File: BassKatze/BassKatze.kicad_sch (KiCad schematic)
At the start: 42 parts, among them U1 ESP32-WROOM-32D

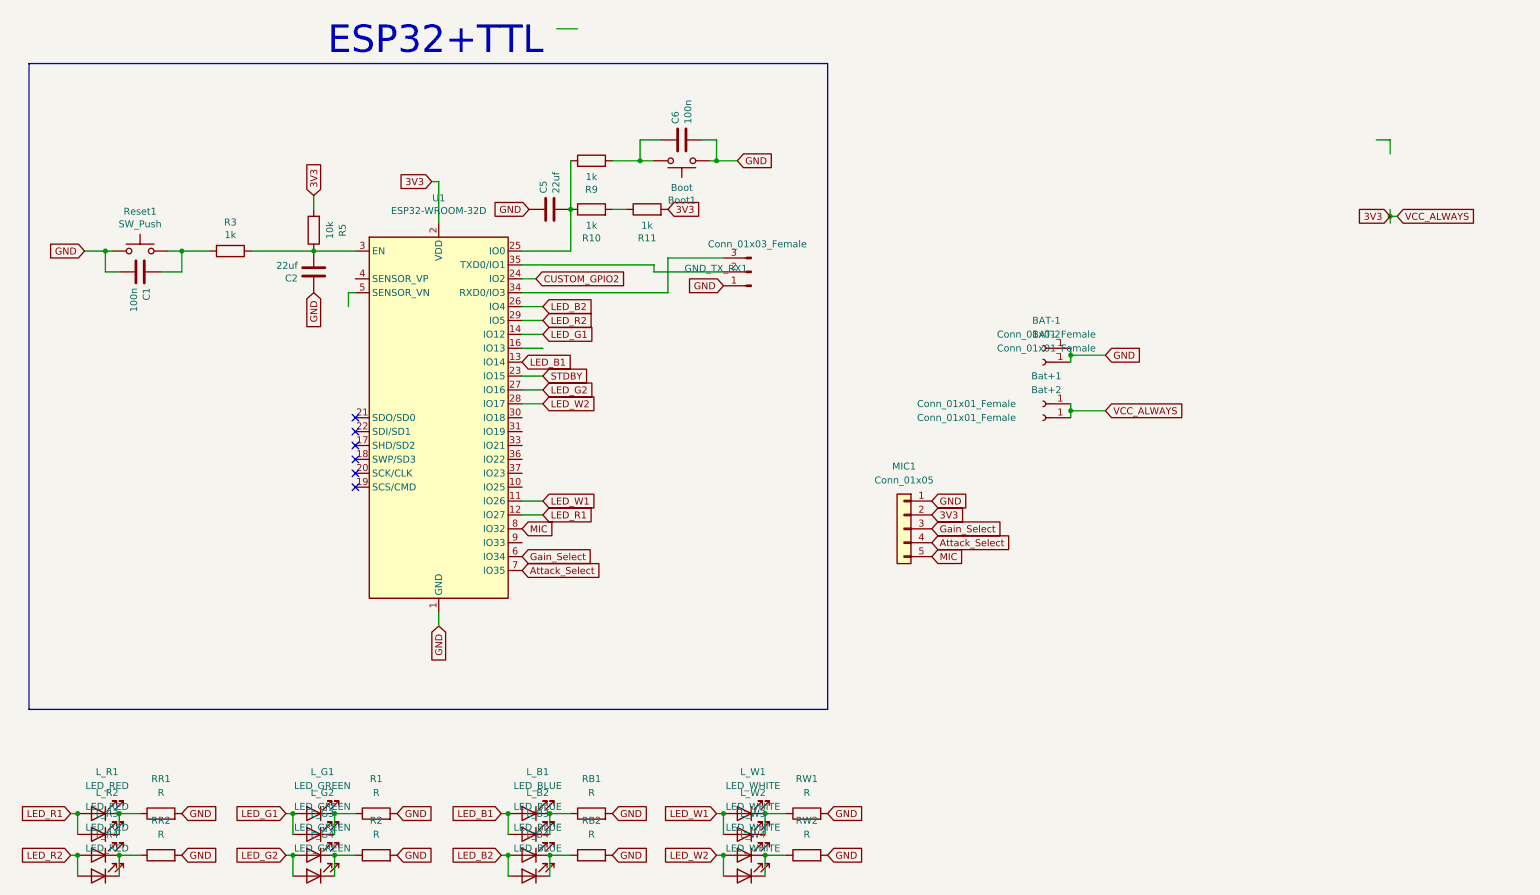
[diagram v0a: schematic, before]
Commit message: esp32 version
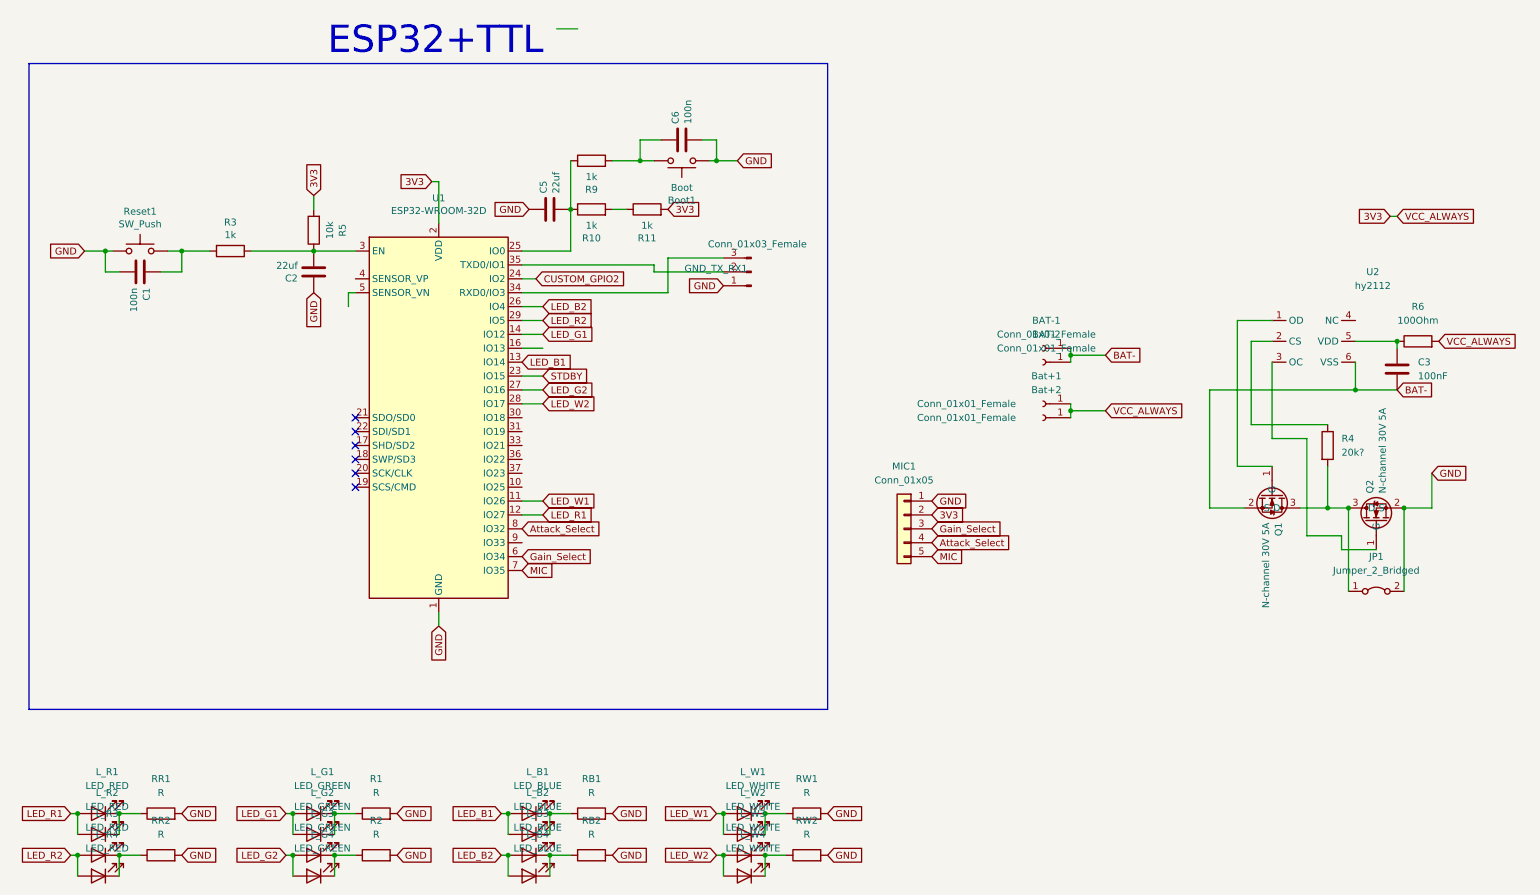
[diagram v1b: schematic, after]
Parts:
- added C3: 100nF, Capacitor_SMD:C_0603_1608Metric, symbol Device:C
- added JP1: Jumper_2_Bridged, Jumper:SolderJumper-2_P1.3mm_Bridged_RoundedPad1.0x1.5mm, symbol Jumper:Jumper_2_Bridged
- added Q1, Q2: N-channel 30V 5A, Package_TO_SOT_SMD:SOT-23, symbol ESP32-DEVKITC-32D:SL2300
- added R4: 20k?, Resistor_SMD:R_0603_1608Metric, symbol Device:R
- added R6: 100Ohm, Resistor_SMD:R_0603_1608Metric, symbol Device:R
- added U2: hy2112, Package_TO_SOT_SMD:SOT-23-6_Handsoldering, symbol hy2112:hy2112
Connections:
- net 3V3: now also R6.2
- net Attack_Select: now also U1.8 (IO32); no longer U1.7 (IO35)
- net GND: now also JP1.2 (B), Q2.2 (S); no longer BAT-1.1 (Pin_1), BAT-2.1 (Pin_1)
- net MIC: now also U1.7 (IO35); no longer U1.8 (IO32)
- new net: JP1.1 (A), Q1.3 (D), Q2.3 (D), R4.2
- new net: Q2.1 (G), U2.3 (OC)
- new net: Q1.1 (G), U2.1 (OD)
- new net: R4.1, U2.2 (CS)
- new net: C3.1, R6.1, U2.5 (VDD)
- new net BAT-: BAT-1.1 (Pin_1), BAT-2.1 (Pin_1), C3.2, Q1.2 (S), U2.6 (VSS)
